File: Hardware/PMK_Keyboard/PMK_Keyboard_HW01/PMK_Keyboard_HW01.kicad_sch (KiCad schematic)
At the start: 0 parts

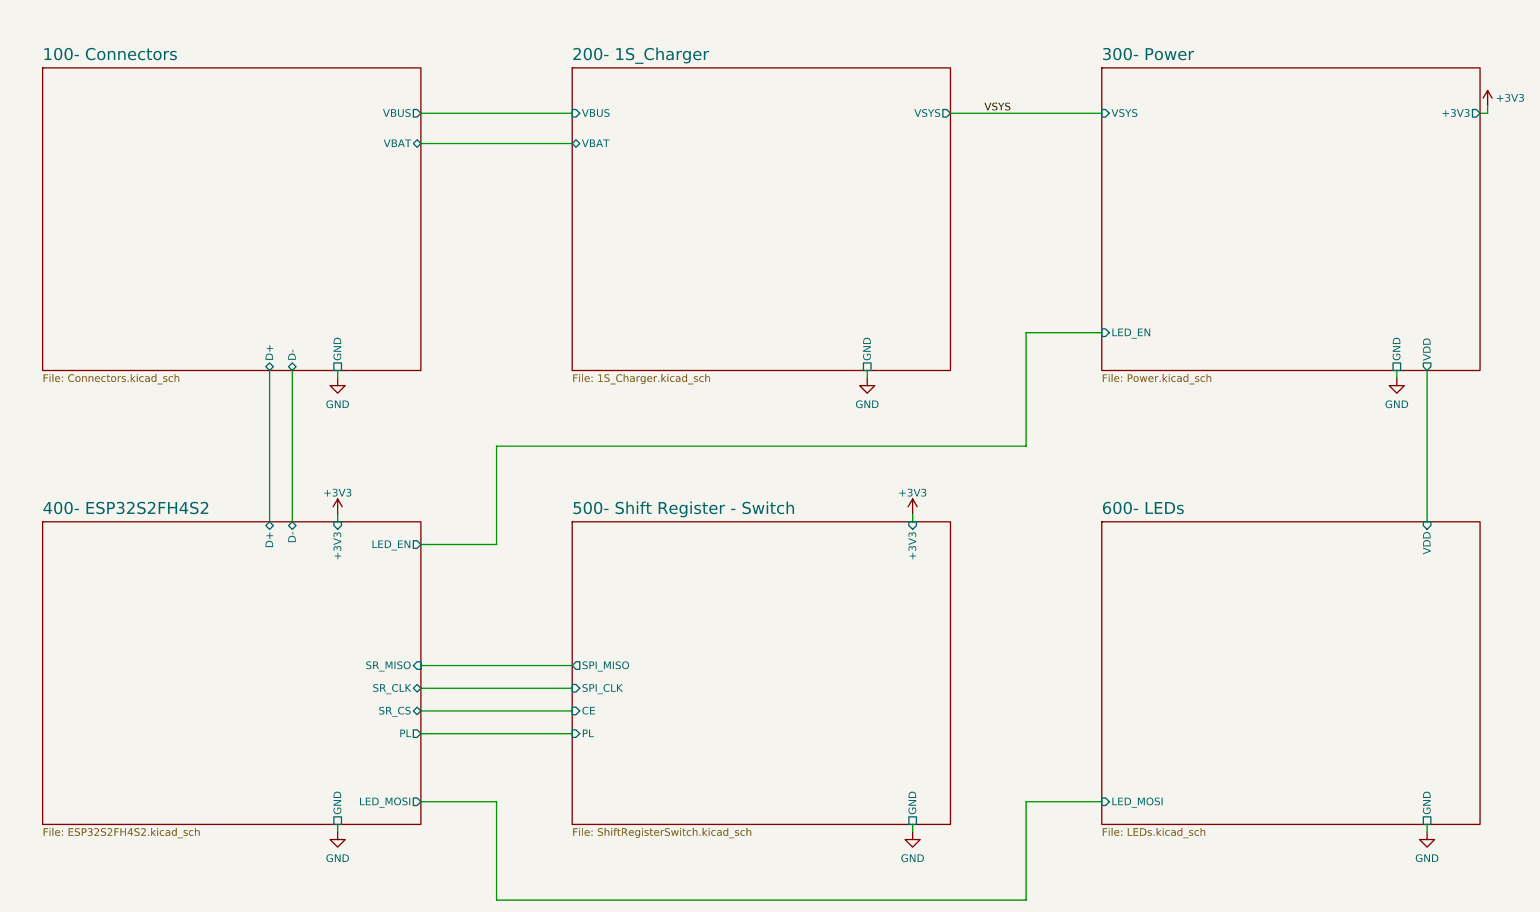
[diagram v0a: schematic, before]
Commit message: started keyboard HW01
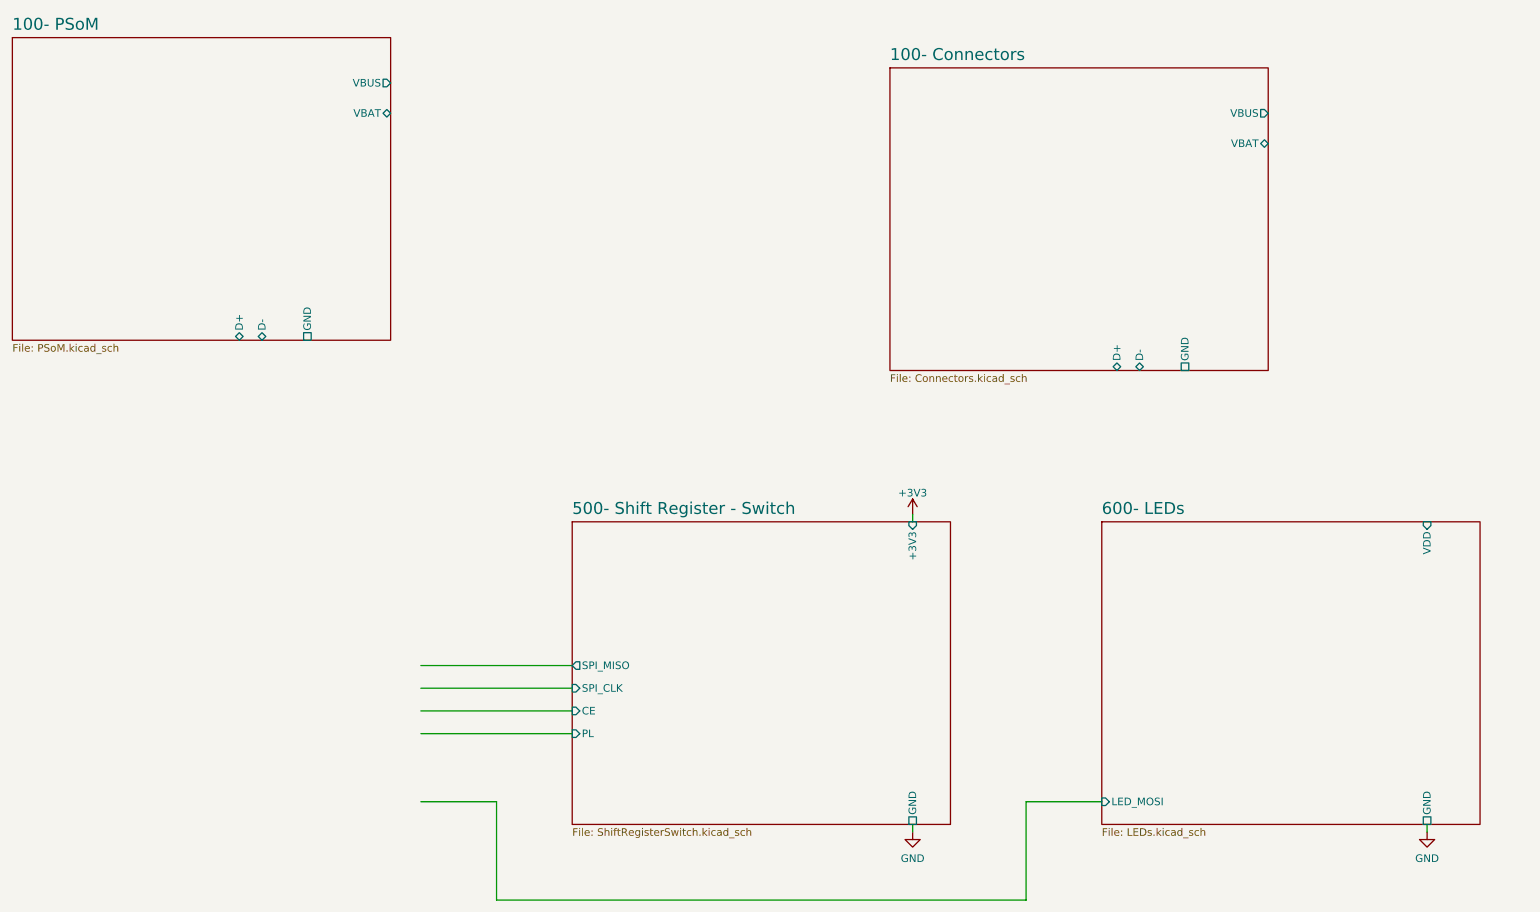
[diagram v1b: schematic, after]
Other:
- removed sheet 200- 1S_Charger
- removed sheet 300- Power
- removed sheet 400- ESP32S2FH4S2
- added sheet 100- PSoM (PSoM.kicad_sch)
